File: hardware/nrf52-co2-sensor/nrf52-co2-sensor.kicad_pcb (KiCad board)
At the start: 4 copper layers, 34 x 15.5 mm, 27 parts, among them J1 USB4105-GF-A, J2 SCD30, J3 Conn_01x02, J4 SWD, SW1 SW_Push, U1 USBLC6-2P6, U2 MDBT50Q-1MV2

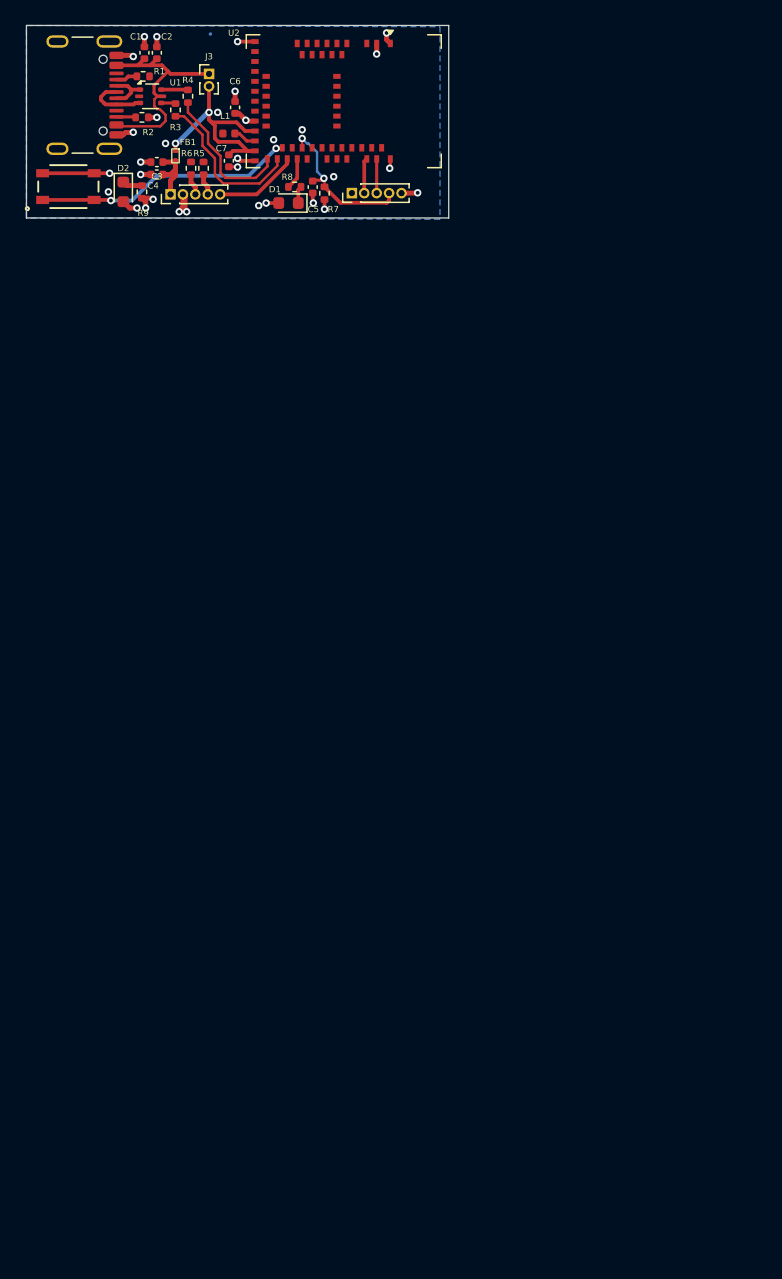
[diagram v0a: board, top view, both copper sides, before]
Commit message: Finished PCB Layout and BOM read for review
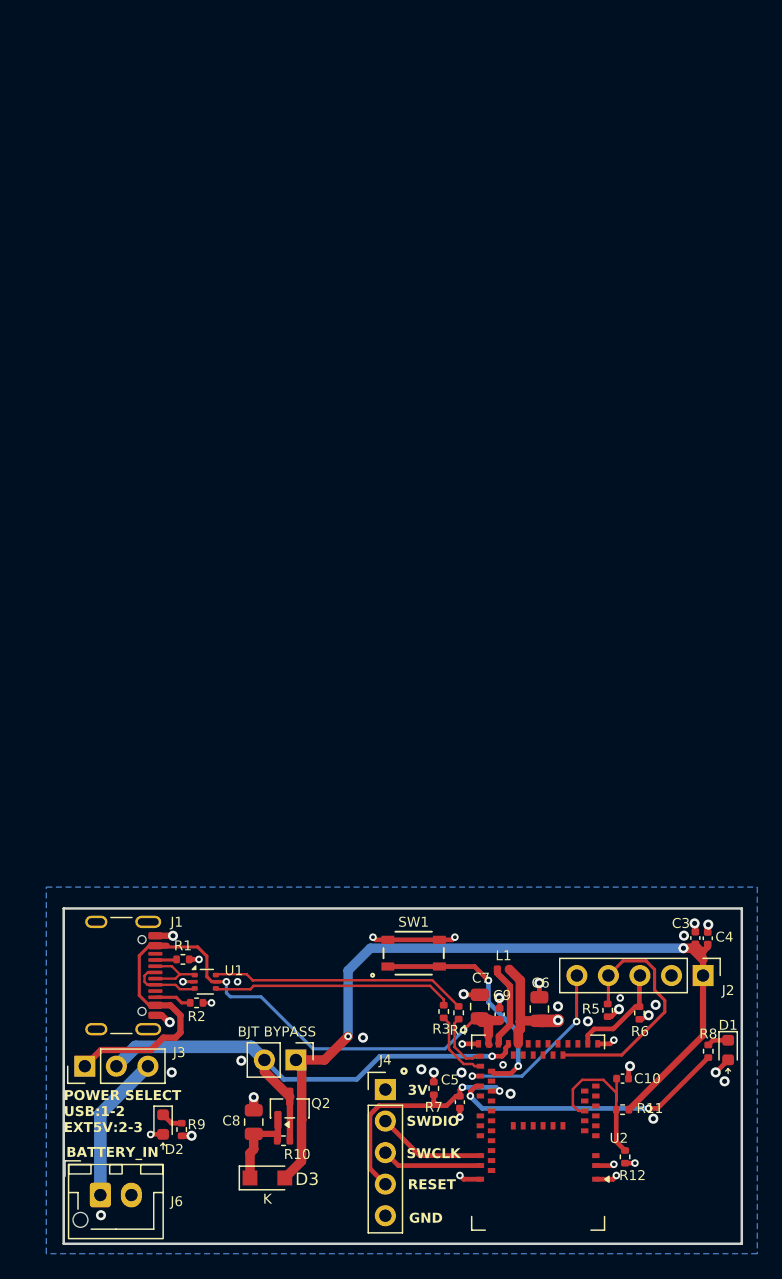
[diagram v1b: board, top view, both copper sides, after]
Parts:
- removed C1: 0.1uf, Capacitor_SMD:C_0402_1005Metric
- removed C2: 10uf, Capacitor_SMD:C_0402_1005Metric
- removed FB1: 600 @ 100Mhz, nrf52-co2-sensor:BLM15AX601SN1D
- added C10: 10nf, Capacitor_SMD:C_0402_1005Metric, F.Cu at (140.5, 160.8)
- added C8: 47uf, Capacitor_SMD:C_0805_2012Metric, F.Cu at (110.8, 164.3)
- added C9: 0.1uf, Capacitor_SMD:C_0402_1005Metric, F.Cu at (130.6, 155.6)
- added D3: 1N914, Diode_SMD:Nexperia_CFP3_SOD-123W, F.Cu at (111.9, 168.8)
- added J6: Conn_01x02, Connector_JST:JST_XH_B2B-XH-AM_1x02_P2.50mm_Vertical, F.Cu at (98.5, 170.2)
- added J7: Conn_01x02, Connector_PinHeader_2.54mm:PinHeader_1x02_P2.54mm_Vertical, F.Cu at (114.2, 159.3)
- added Q2: Q_NPN_BEC, Package_TO_SOT_SMD:SOT-23, F.Cu at (113.7, 163.2)
- added R10: 150, Resistor_SMD:R_0402_1005Metric, F.Cu at (113.2, 165.8)
- added R11: 2.2M, Resistor_SMD:R_0402_1005Metric, F.Cu at (140.5, 163.3)
- added R12: 1M, Resistor_SMD:R_0402_1005Metric, F.Cu at (140.7, 167.1)
- C6, C7: footprint Capacitor_SMD:C_0402_1005Metric -> Capacitor_SMD:C_0805_2012Metric
- J2, J4: footprint Connector_PinHeader_1.00mm:PinHeader_1x05_P1.00mm_Vertical -> Connector_PinHeader_2.54mm:PinHeader_1x05_P2.54mm_Vertical
- J3: value Conn_01x02 -> Conn_01x03; footprint Connector_PinHeader_1.00mm:PinHeader_1x02_P1.00mm_Vertical -> Connector_PinHeader_2.54mm:PinHeader_1x03_P2.54mm_Vertical
- R8: value 4.7k -> 2.2k
- moved U2 84.5 mm to (133.7, 165.2), turned to 180 degrees
- moved J3 80.5 mm to (97.2, 159.8), turned to 90 degrees
- moved R8 77.2 mm to (147.4, 158.6), turned to -90 degrees
- moved R6 77.0 mm to (141.9, 155.5), turned to -90 degrees
- moved R4 77.0 mm to (127.3, 155.5)
- moved D1 76.8 mm to (149.0, 158.5), turned to -90 degrees
- moved C6 76.6 mm to (133.8, 155.2)
- moved J2 76.1 mm to (147.0, 152.5), turned to -90 degrees
- moved C3 76.1 mm to (146.4, 149.5), turned to 90 degrees
- moved C4 75.8 mm to (147.4, 149.5), turned to 90 degrees
- moved R3 75.7 mm to (126.1, 155.4)
- moved R9 75.6 mm to (105.0, 164.9)
- moved R5 75.2 mm to (139.3, 155.3), turned to -90 degrees
- moved D2 75.2 mm to (103.5, 164.5)
- moved C5 74.6 mm to (127.4, 162.7)
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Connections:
- net /D+_MCU renamed /D_MCU+
- net /D-_MCU renamed /D_MCU-
- net /GPIO P0.13 renamed /SCD30_RDY
- net /GPIO P0.14 renamed /BUTTON_1
- net /GPIO P0.15 renamed /LED_1
- net /VBUS_SENS renamed /POWER_SENS
- net Net-(J1-CC1) renamed /CC1
- net Net-(J1-CC2) renamed /CC2
- net Net-(R3-Pad2) renamed /D1+
- net Net-(R4-Pad1) renamed /D1-
- J1 pad A4: /VBUS_USB -> /VBUS
- J1 pad A9: /VBUS_USB -> /VBUS
- J1 pad B4: /VBUS_USB -> /VBUS
- J1 pad B9: /VBUS_USB -> /VBUS
- J2 pad 3: /SCL -> /SCD30_SCL
- J2 pad 4: /SDA -> /SCD30_SDA
- J3 pad 1: /VBUS_USB -> /VBUS
- J3 pad 2: /VBUS -> /POWER_RAW
- R5 pad 1: /SDA -> /SCD30_SDA
- R6 pad 1: /SCL -> /SCD30_SCL
- U1 pad 5: /VBUS_USB -> /VBUS
- U2 pad 16: unconnected-(U2B-P0.27-Pad16) -> /SCD30_SCL
- U2 pad 19: unconnected-(U2B-P0.26-Pad19) -> /SCD30_SDA
- U2 pad 30: /VBUS -> /POWER_RAW
- U2 pad 9: unconnected-(U2B-P0.03/AINI-Pad9) -> /POWER_ADC
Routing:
- net /POWER_SENS: track 5.15 -> 67.1 mm, vias 0 -> 2
- net /POWER_RAW: track 0.00 -> 43.6 mm, vias 0 -> 1
- net /VBUS: track 20.6 -> 54.7 mm
- net /SCD30_SDA: track 0.00 -> 20.2 mm
- net /LED_1: track 2.54 -> 22.6 mm, vias 0 -> 2
- net /VBUS_USB: track 19.0 -> 0.00 mm
- net /D1-: track 2.16 -> 20.7 mm
- net /D1+: track 1.17 -> 19.4 mm
- net /POWER_ADC: track 0.00 -> 13.4 mm
- net /External Power: track 0.00 -> 12.0 mm
- net /3V_VDD: track 4.96 -> 14.8 mm, vias 4 -> 6
- net /SCD30_SCL: track 0.00 -> 8.32 mm
- net /SCD30_RDY: track 6.84 -> 14.6 mm, vias 0 -> 2
- net /RESETN: track 12.6 -> 20.0 mm
- net /BASE: track 0.00 -> 7.33 mm
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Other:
- board size 34 x 15.5 mm -> 54.6 x 27 mm
- rule pad_to_mask_clearance: 0 -> 0.0381
- board text added: "3V"
- board text added: "BATTERY_IN"
- board text added: "BJT BYPASS"
- board text added: "GND"
- board text added: "POWER SELECT USB:1-2 EXT5V:2-3"
- board text added: "RESET"
- board text added: "SWCLK"
- board text added: "SWDIO"
